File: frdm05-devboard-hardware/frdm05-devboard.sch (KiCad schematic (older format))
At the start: 63 parts, among them CON1 MIKROBUS_HOST_CONN, J1 SD_Card_Fix, J2 KEYBOARD, J3 Conn_01x06, J4 LIGHT SENSOR, J5 1602 LCD VIA I2C, Q1 BCV62, Q2 BC817, SW1 PTS810, SW2 PTS810, SW3 PTS810, SW4 PTS810, SW5 PTS810, SW6 PTS810, U1 25LCxxx, U2 PCF8563T, U3 LM75C, U4 T24C02A, U5 T24C02A, U6 74HCT1G125GV, Y1 32768Hz

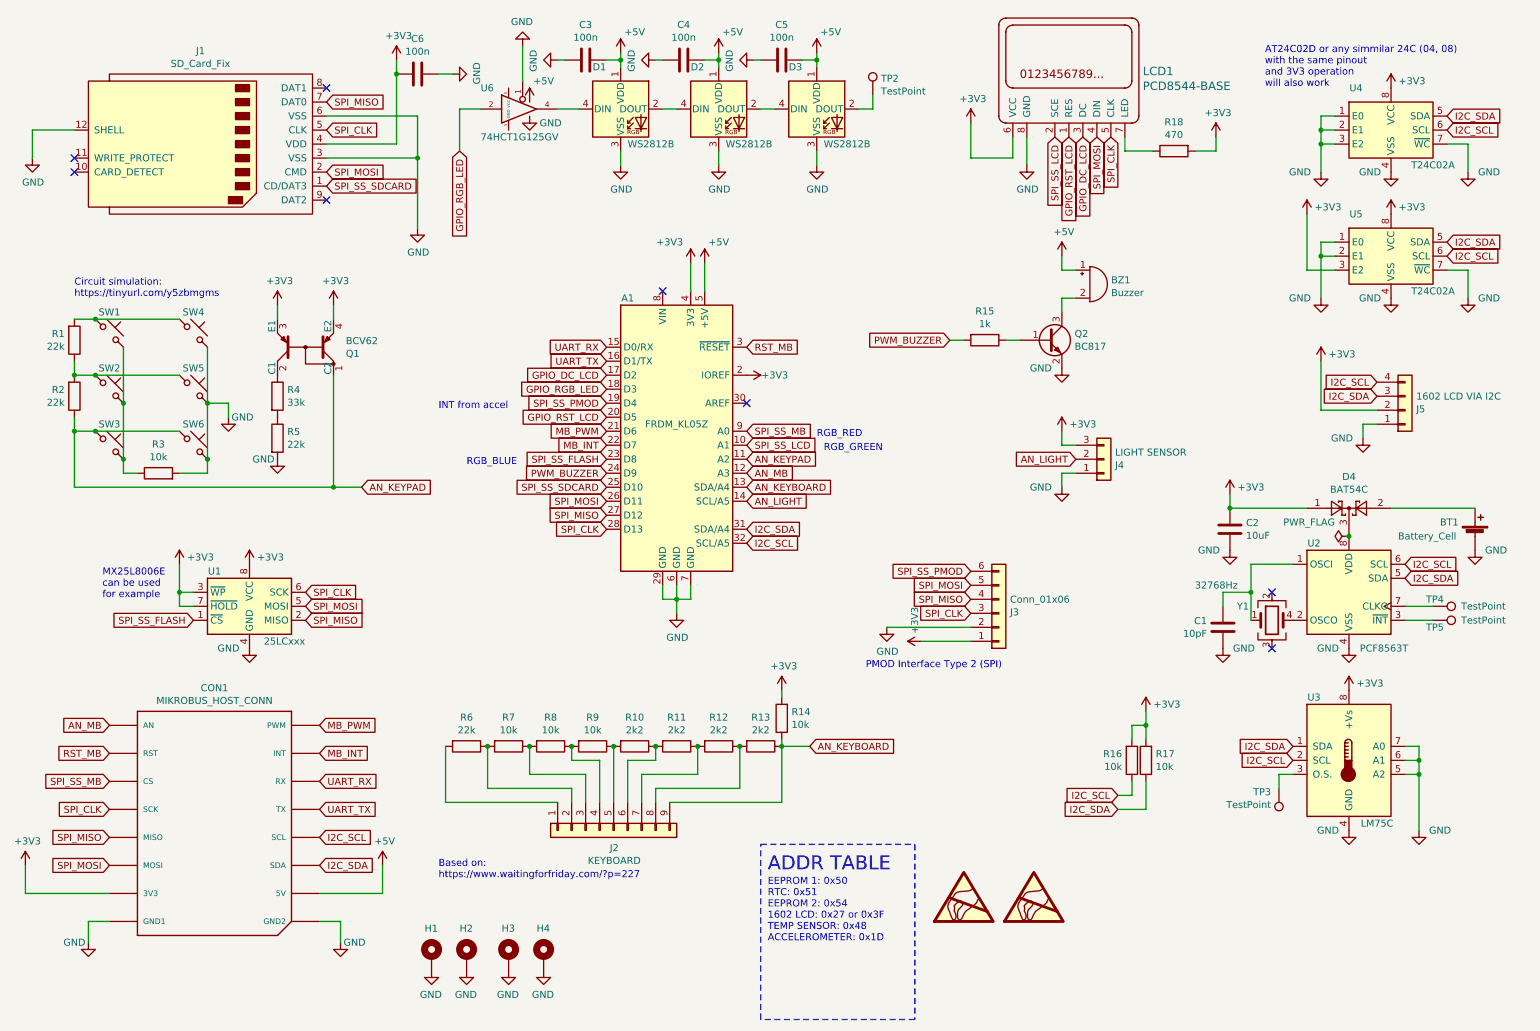
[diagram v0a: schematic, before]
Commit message: Initial commit of Rev.2 hardware
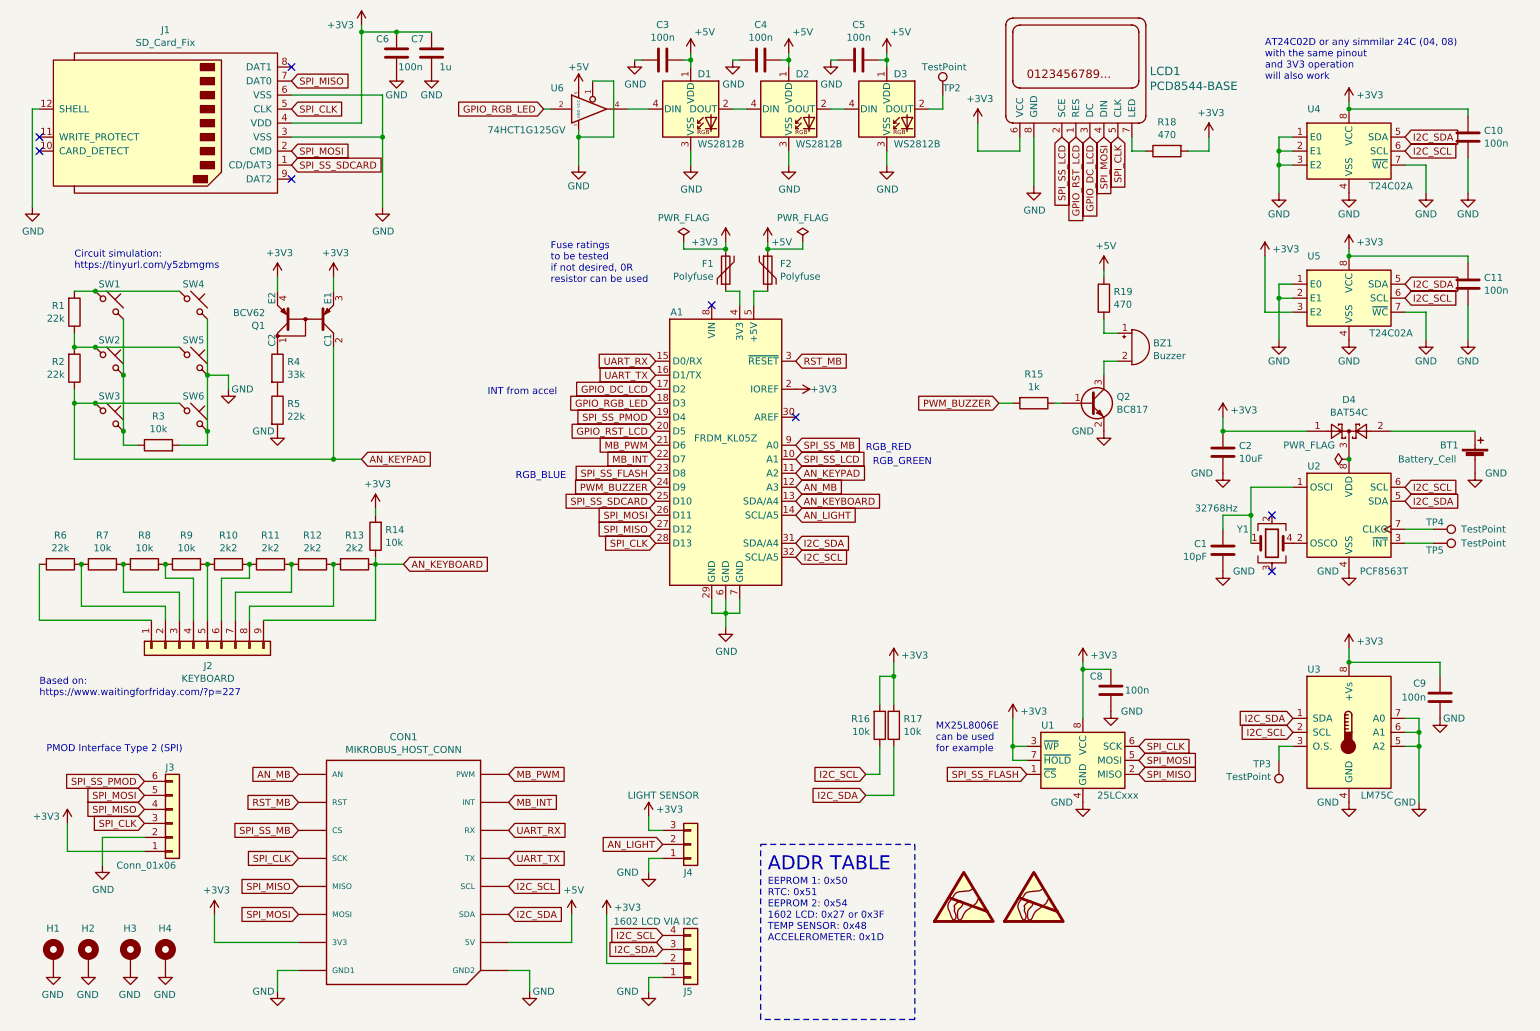
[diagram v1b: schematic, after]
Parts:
- added C10, C11, C8, C9: 100n, Capacitor_SMD:C_0805_2012Metric_Pad1.18x1.45mm_HandSolder, symbol Device:C
- added C7: 1u, Capacitor_SMD:C_0805_2012Metric_Pad1.18x1.45mm_HandSolder, symbol Device:C
- added F1, F2: Polyfuse, Fuse:Fuse_0805_2012Metric, symbol Device:Polyfuse
- added R19: 470, Resistor_SMD:R_0805_2012Metric_Pad1.20x1.40mm_HandSolder, symbol Device:R
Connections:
- net +3V3: now also C10.2, C11.2, C7.2, C8.1, C9.2, F1.2; no longer A1.4 (3V3)
- net +5V: now also U6.5 (VCC), F2.1, R19.1; no longer A1.5 (+5V), BZ1.1 (-)
- net AN_KEYPAD: now also Q1.2 (C1); no longer Q1.1 (C2)
- net GND: now also U6.3 (GND), C10.1, C11.1, C7.1, C8.2, C9.1
- net at R4.1: now also Q1.1 (C2); no longer Q1.2 (C1)
- new net: BZ1.1 (-), R19.2
- new net: A1.4 (3V3), F1.1
- new net: A1.5 (+5V), F2.2
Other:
- note added: "Fuse ratings\nto be tested\nif not desired, 0R\nresistor can be used"
- moved on the sheet: A1, BT1, BZ1, C1, C2, C3, C4, C5, C6, CON1, D1, D2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
